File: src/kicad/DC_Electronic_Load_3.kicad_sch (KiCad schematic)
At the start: 12 parts, among them IC1 LM393D, IC2 TL072D, U1 AD8628, U2 AD8628, U3 AD8628, U4 SN74AHC08

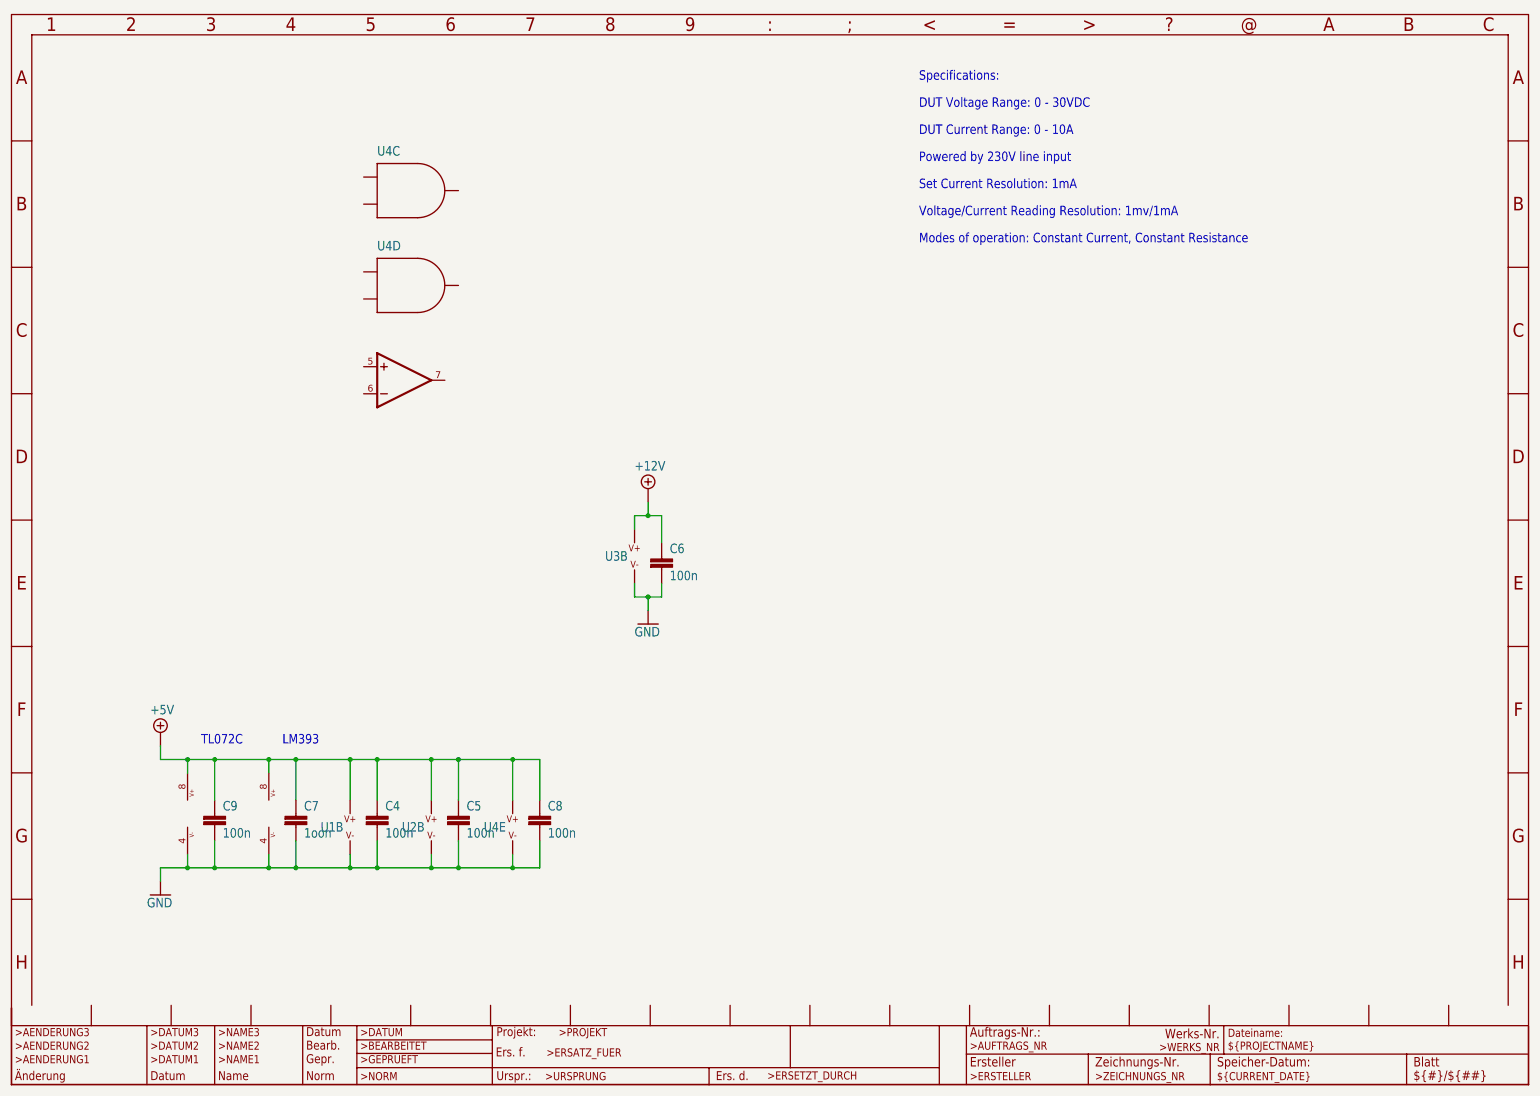
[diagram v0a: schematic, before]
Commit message: Tidy up kicad schematic
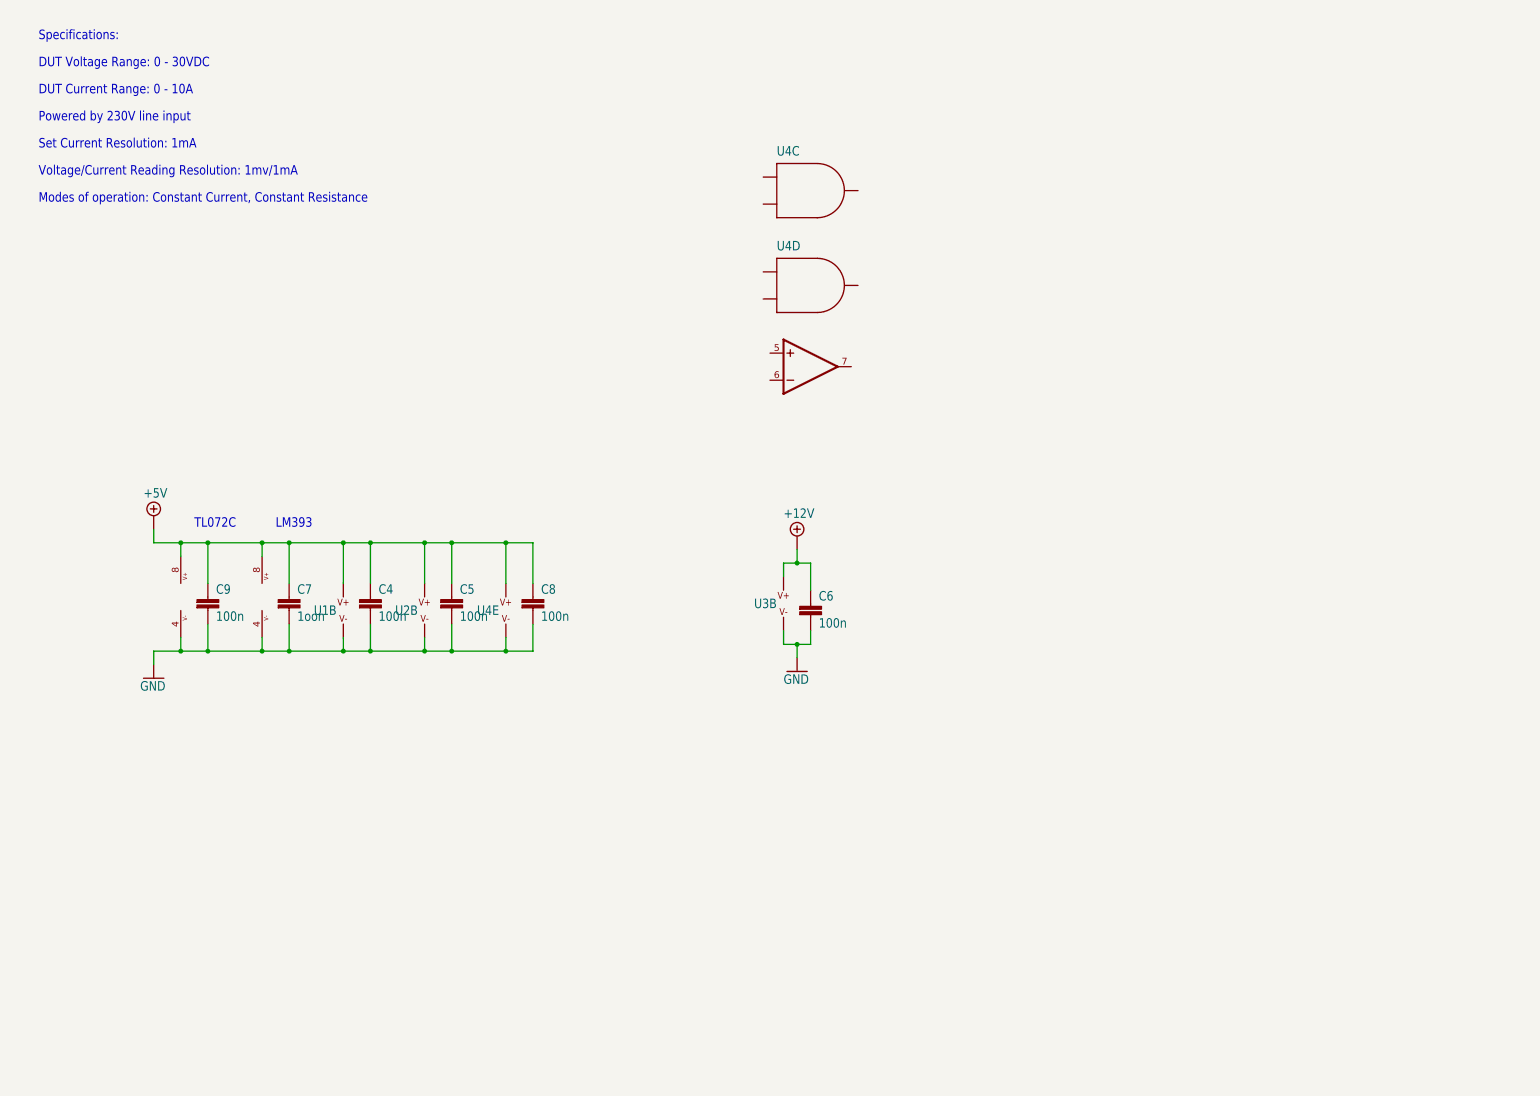
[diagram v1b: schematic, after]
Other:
- title: (none) -> DC Electronic Load
- moved on the sheet: C4, C5, C6, C7, C8, C9, U1B, U2B, U3B, U4C, U4D, U4E
